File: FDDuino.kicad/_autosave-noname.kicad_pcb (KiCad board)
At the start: 2 copper layers, 7 parts, among them P1 RASPI_V2, P3 LS04, P5 LS04, P7 MSX_SLOT, U1 74LS74, U2 7400, U3 74F676

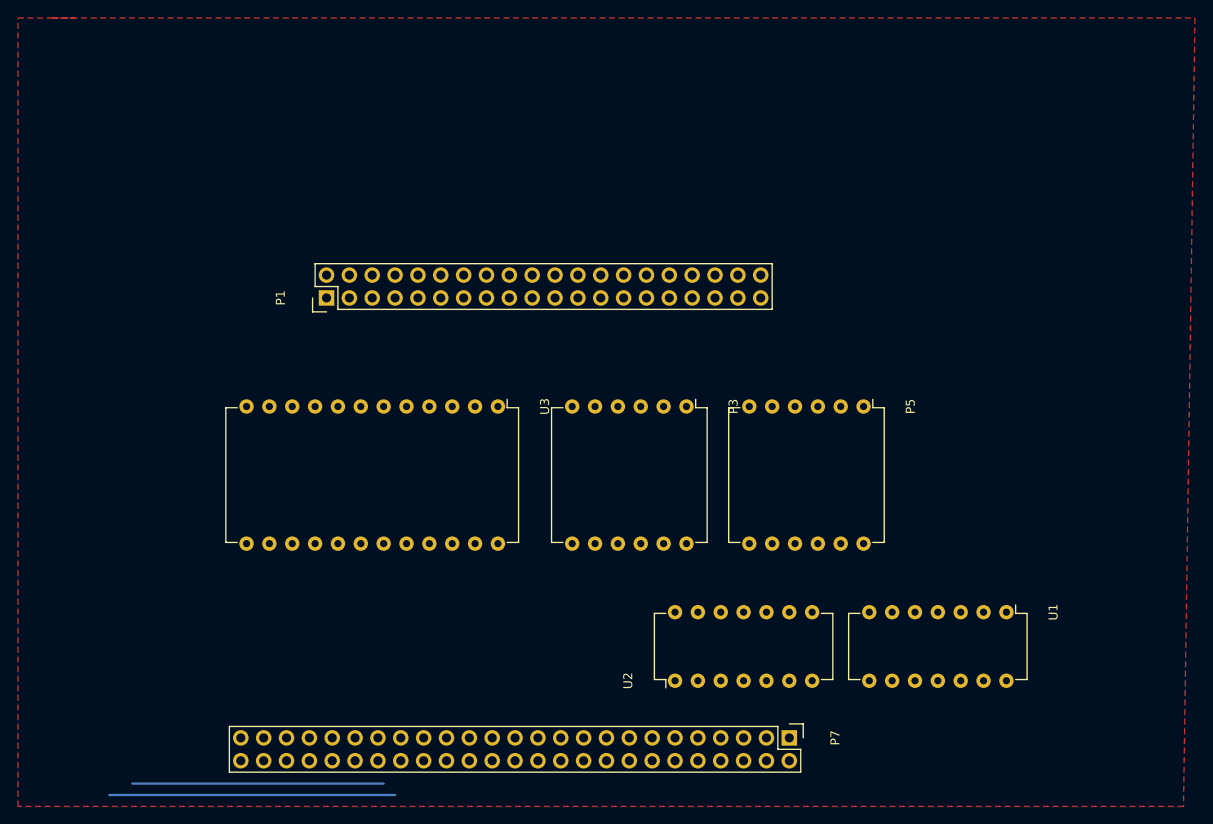
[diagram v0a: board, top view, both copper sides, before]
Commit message: FDDuino schematic update
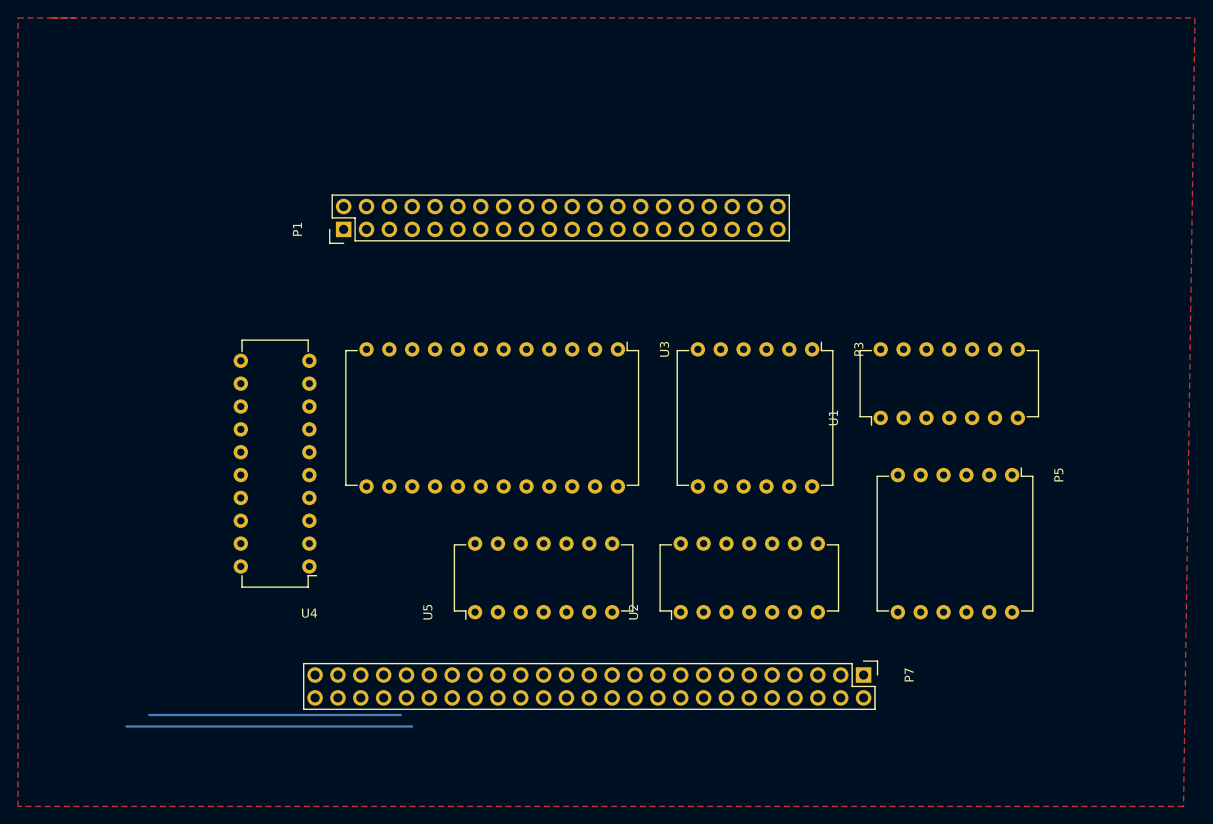
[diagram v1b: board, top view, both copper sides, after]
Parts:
- added U4: 74LS245, Housings_DIP:DIP-20_W7.62mm, F.Cu at (127.6, 120.7)
- added U5: 74LS00, Housings_DIP:DIP-14_W7.62mm, F.Cu at (146.1, 125.7)
- moved U1 25.7 mm to (191.1, 104.1), turned to 90 degrees
- moved P5 18.2 mm to (205.7, 110.5)
- moved P3 15.3 mm to (183.5, 96.5)
- moved U3 14.8 mm to (161.9, 96.5)
- moved P7 10.8 mm to (189.2, 132.7)
- moved P1 7.85 mm to (131.4, 83.2)
- moved U2 7.65 mm to (168.9, 125.7)
